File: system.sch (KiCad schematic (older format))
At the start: 1 part

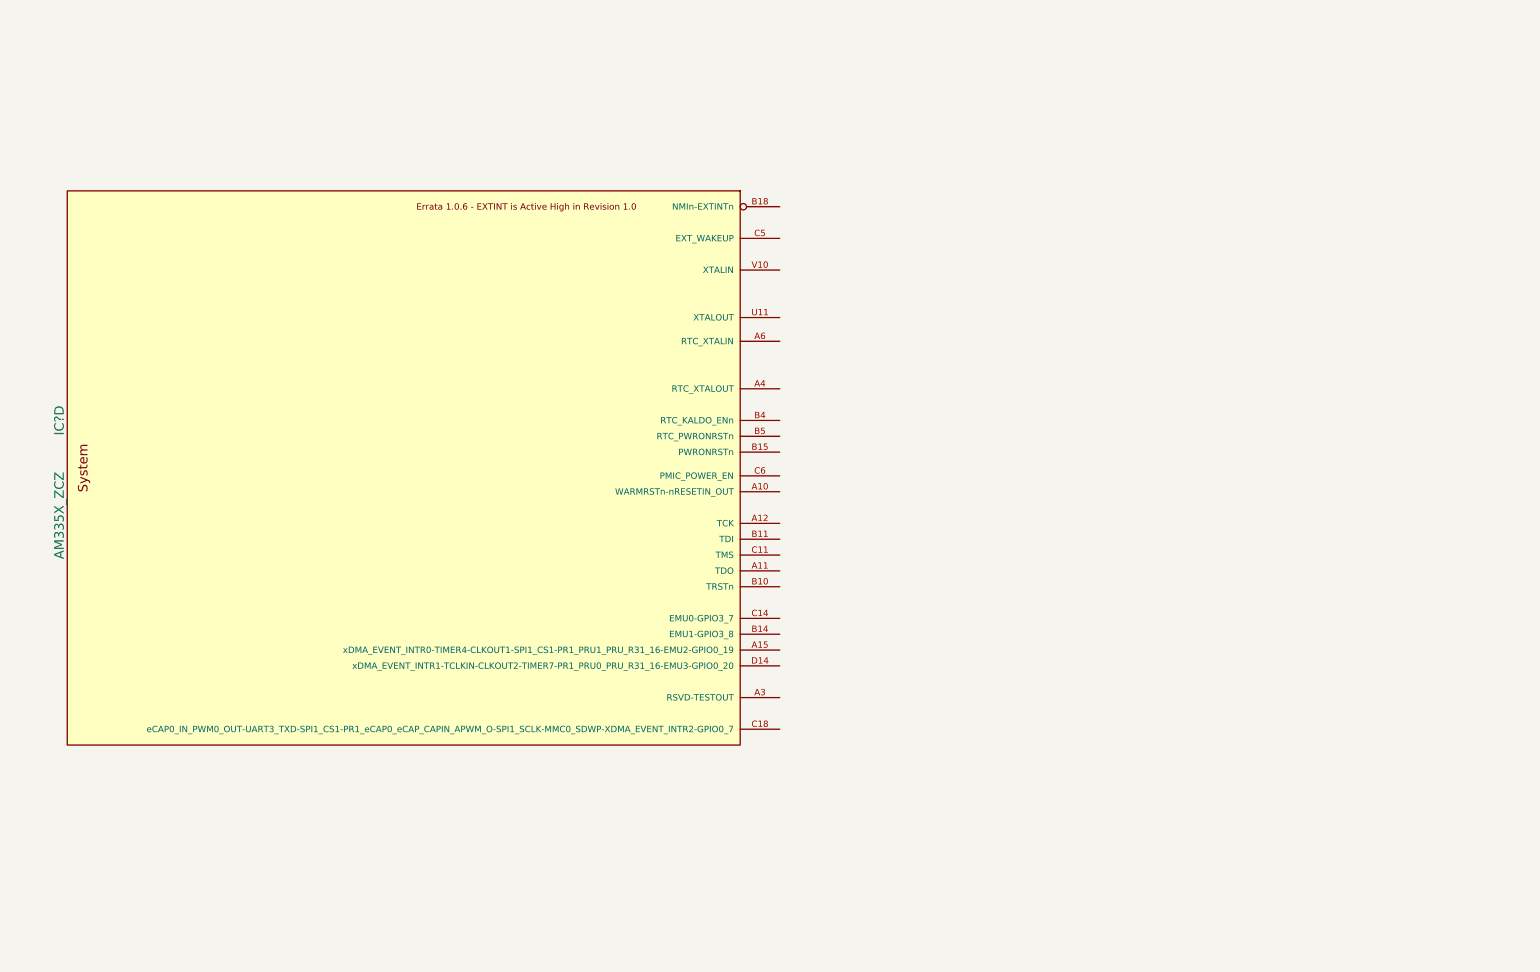
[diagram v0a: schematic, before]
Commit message: system sheet
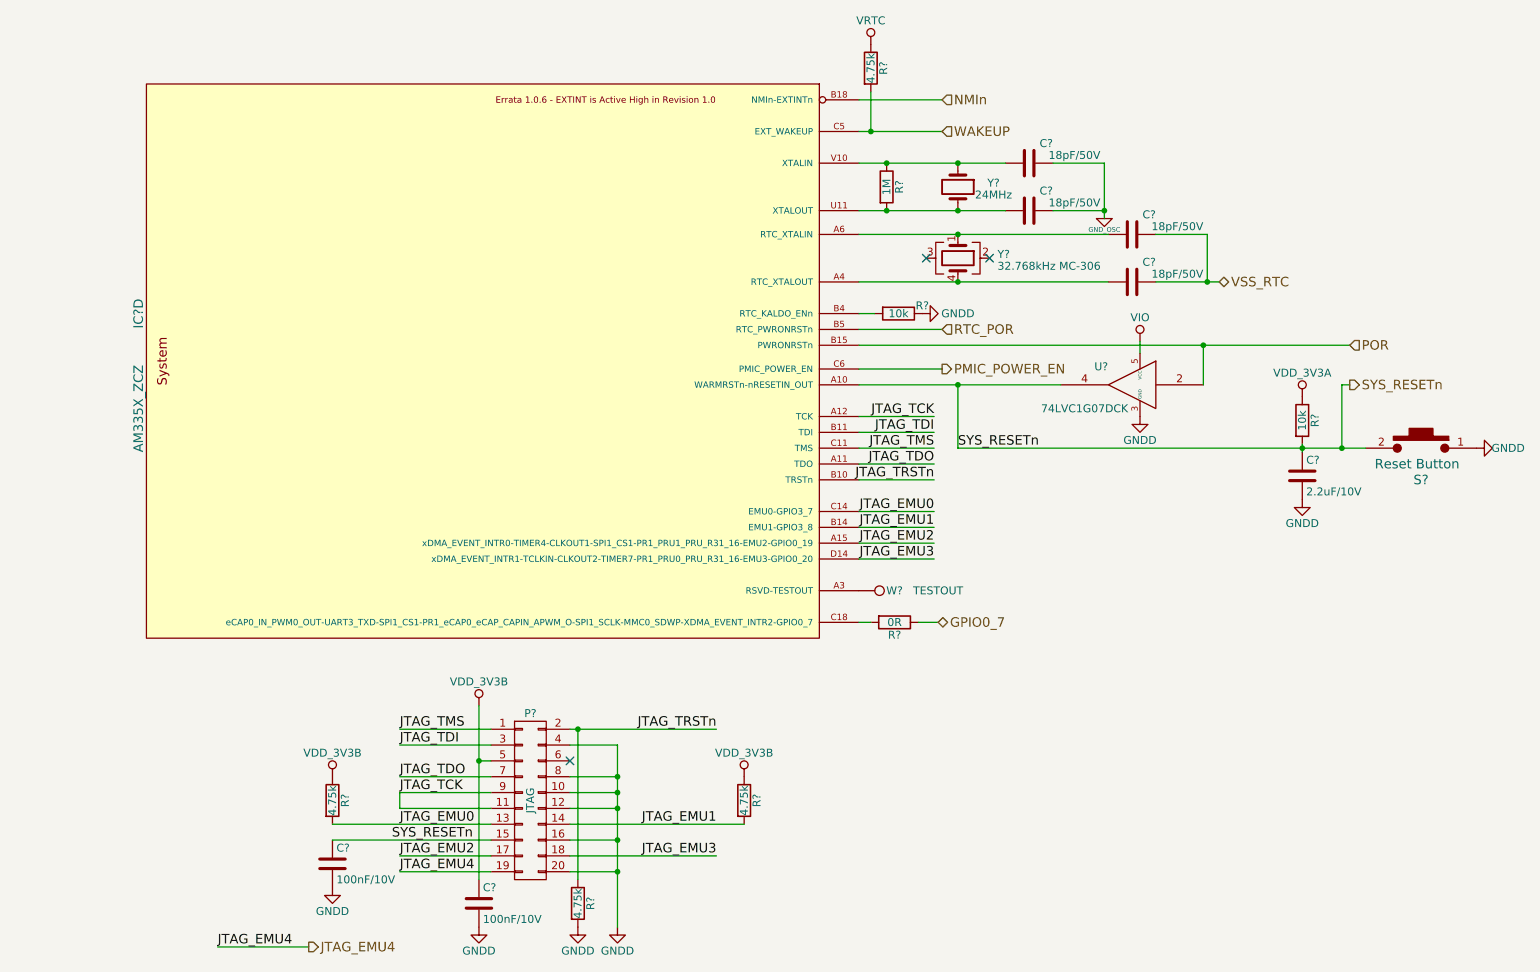
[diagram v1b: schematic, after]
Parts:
- added C? (x4): 18pF/50V, symbol C
- added C?: 2.2uF/10V, symbol C
- added C? (x2): 100nF/10V, symbol C
- added P?: JTAG, symbol CONN_02X10
- added R? (x4): 4.75k, symbol R
- added R?: 1M, symbol R
- added R? (x2): 10k, symbol R
- added R?: 0R, symbol R
- added S?: Reset Button, symbol PushButton
- added U?: 74LVC1G07DCK, symbol 74LVC1G07DCK
- added W?: TESTOUT, symbol TEST_1P
- added Y?: 24MHz, symbol Crystal
- added Y?: 32.768kHz MC-306, symbol Crystal_GND23
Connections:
- net SYS_RESETn: now reaches IC?.A10 (WARMRSTn-nRESETIN_OUT)
- net SYS_RESETn: now also C?.1, C?.1, P?.15 (P15), R?.2, S?.2, U?.4
- net JTAG_TDO: now reaches IC?.A11 (TDO)
- net JTAG_TDO: now also P?.7 (P7)
- net JTAG_TCK: now reaches IC?.A12 (TCK)
- net JTAG_TCK: now also P?.11 (P11), P?.9 (P9)
- net JTAG_EMU2: now reaches IC?.A15 (xDMA_EVENT_INTR0-TIMER4-CLKOUT1-SPI1_CS1-PR1_PRU1_PRU_R31_16-EMU2-GPIO0_19)
- net JTAG_EMU2: now also P?.17 (P17)
- net at IC?.A3 (RSVD-TESTOUT): now also W?.1
- net at IC?.A4 (RTC_XTALOUT): now also C?.1, Y?.4
- net at IC?.A6 (RTC_XTALIN): now also C?.1, Y?.1
- net JTAG_TRSTn: now reaches IC?.B10 (TRSTn)
- net JTAG_TRSTn: now also P?.2 (P2), R?.1
- net JTAG_TDI: now reaches IC?.B11 (TDI)
- net JTAG_TDI: now also P?.3 (P3)
- net JTAG_EMU1: now reaches IC?.B14 (EMU1-GPIO3_8)
- net JTAG_EMU1: now also P?.14 (P14), R?.2
- net POR: now reaches IC?.B15 (PWRONRSTn)
- net POR: now also U?.2
- net NMIn: now reaches IC?.B18 (NMIn-EXTINTn)
- net at IC?.B4 (RTC_KALDO_ENn): now also R?.2
- net RTC_POR: now reaches IC?.B5 (RTC_PWRONRSTn)
- net JTAG_TMS: now reaches IC?.C11 (TMS)
- net JTAG_TMS: now also P?.1 (P1)
- net JTAG_EMU0: now reaches IC?.C14 (EMU0-GPIO3_7)
- net JTAG_EMU0: now also P?.13 (P13), R?.2
- net at IC?.C18 (eCAP0_IN_PWM0_OUT-UART3_TXD-SPI1_CS1-PR1_eCAP0_eCAP_CAPIN_APWM_O-SPI1_SCLK-MMC0_SDWP-XDMA_EVENT_INTR2-GPIO0_7): now also R?.2
- net WAKEUP: now reaches IC?.C5 (EXT_WAKEUP)
- net WAKEUP: now also R?.2
- net PMIC_POWER_EN: now reaches IC?.C6 (PMIC_POWER_EN)
- net JTAG_EMU3: now reaches IC?.D14 (xDMA_EVENT_INTR1-TCLKIN-CLKOUT2-TIMER7-PR1_PRU0_PRU_R31_16-EMU3-GPIO0_20)
- net JTAG_EMU3: now also P?.18 (P18)
- net at IC?.U11 (XTALOUT): now also C?.1, R?.2, Y?.2
- net at IC?.V10 (XTALIN): now also C?.1, R?.1, Y?.1
- new net GNDD: C?.2, C?.2, C?.2, P?.10 (P10), P?.12 (P12), P?.16 (P16), P?.20 (P20), P?.4 (P4), P?.8 (P8), R?.1, R?.2, S?.1, U?.3 (GND)
- new net GND_OSC: C?.2, C?.2
- new net GPIO0_7: R?.1
- new net JTAG_EMU4: P?.19 (P19)
- new net VDD_3V3A: R?.1
- new net VDD_3V3B: C?.1, P?.5 (P5), R?.1, R?.1
- new net VIO: U?.5 (VCC)
- new net VRTC: R?.1
- new net VSS_RTC: C?.2, C?.2
- no-connect marks 0 -> 3
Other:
- moved on the sheet: IC?D
